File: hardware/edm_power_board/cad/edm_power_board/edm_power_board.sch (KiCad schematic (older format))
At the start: 0 parts

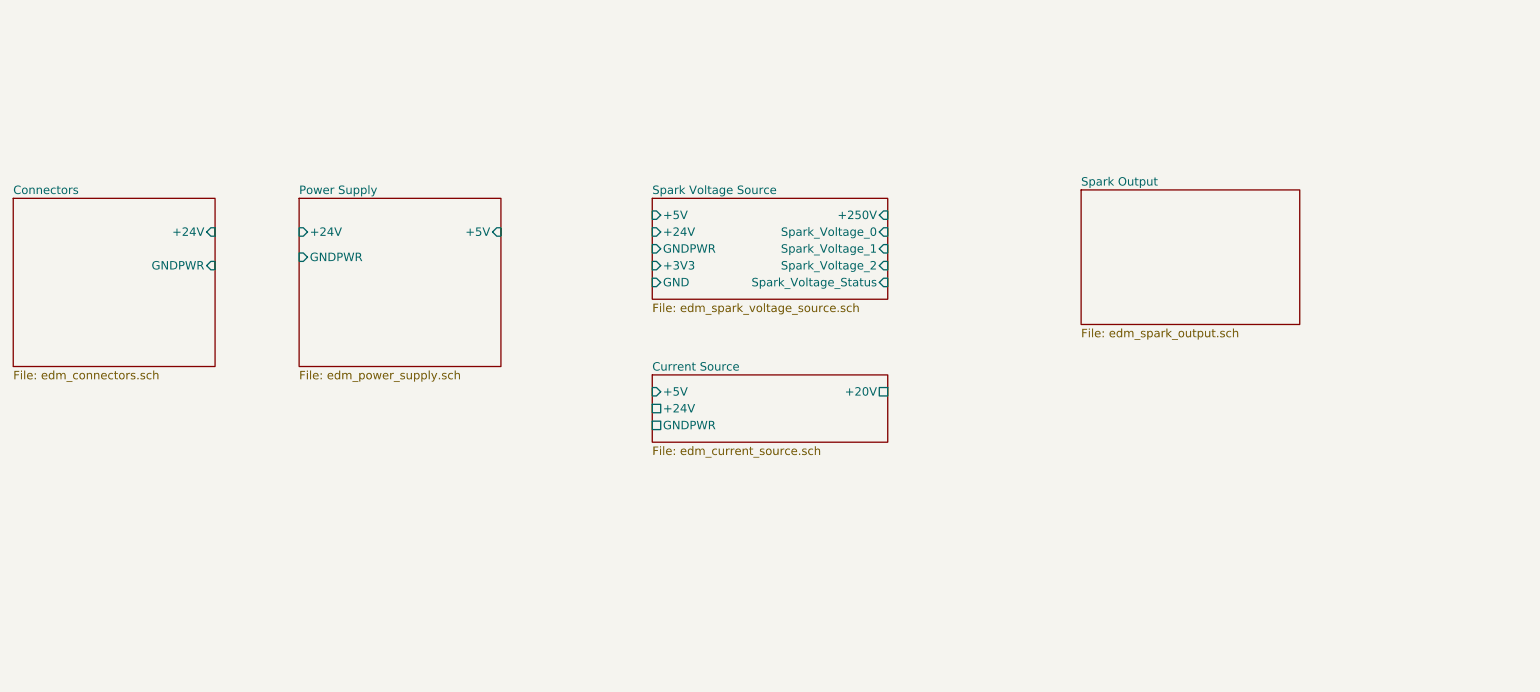
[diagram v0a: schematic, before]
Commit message: Interconnections
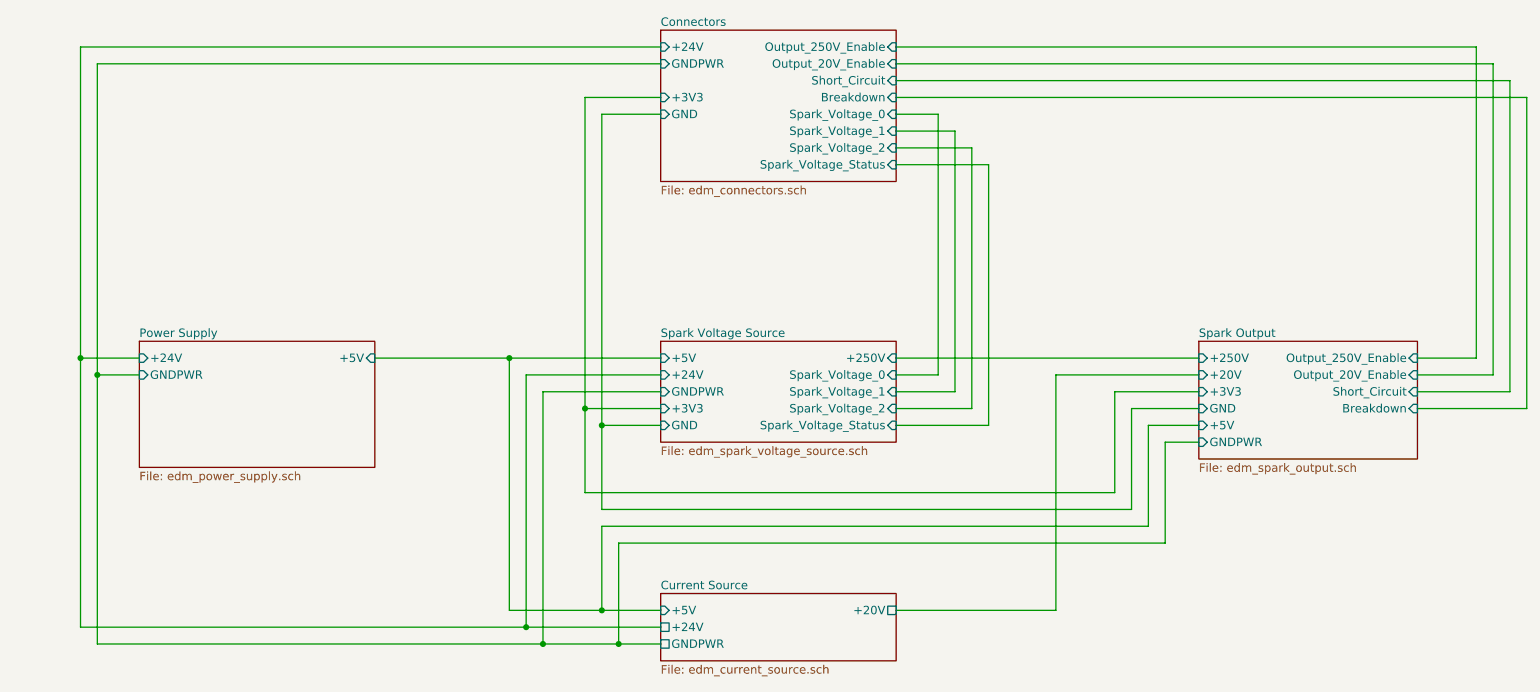
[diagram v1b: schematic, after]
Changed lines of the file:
@@
 $EndDescr
 $Sheet
-S 5000 3750 1400 400
+S 5050 5050 1400 400
 U 5A71F0AB
 F0 "Current Source" 50
 F1 "edm_current_source.sch" 50
-F2 "+24V" U L 5000 3950 50
-F3 "GNDPWR" U L 5000 4050 50
-F4 "+20V" U R 6400 3850 50
-F5 "+5V" I L 5000 3850 50
-$EndSheet
-$Sheet
-S 5000 2700 1400 600
+F2 "+24V" U L 5050 5250 50
+F3 "GNDPWR" U L 5050 5350 50
+F4 "+20V" U R 6450 5150 50
+F5 "+5V" I L 5050 5150 50
+$EndSheet
+$Sheet
+S 5050 3550 1400 600
 U 5A728D61
 F0 "Spark Voltage Source" 50
 F1 "edm_spark_voltage_source.sch" 50
-F2 "+24V" I L 5000 2900 50
-F3 "GNDPWR" I L 5000 3000 50
-F4 "+250V" I R 6400 2800 50
-F5 "+5V" I L 5000 2800 50
-F6 "GND" I L 5000 3200 50
-F7 "+3V3" I L 5000 3100 50
-F8 "Spark_Voltage_0" I R 6400 2900 50
-F9 "Spark_Voltage_1" I R 6400 3000 50
-F10 "Spark_Voltage_2" I R 6400 3100 50
-F11 "Spark_Voltage_Status" I R 6400 3200 50
-$EndSheet
-$Sheet
-S 2900 2700 1200 1000
+F2 "+24V" I L 5050 3750 50
+F3 "GNDPWR" I L 5050 3850 50
+F4 "+250V" I R 6450 3650 50
+F5 "+5V" I L 5050 3650 50
+F6 "GND" I L 5050 4050 50
+F7 "+3V3" I L 5050 3950 50
+F8 "Spark_Voltage_0" I R 6450 3750 50
+F9 "Spark_Voltage_1" I R 6450 3850 50
+F10 "Spark_Voltage_2" I R 6450 3950 50
+F11 "Spark_Voltage_Status" I R 6450 4050 50
+$EndSheet
+$Sheet
+S 1950 3550 1400 750
 U 5A73A880
 F0 "Power Supply" 50
 F1 "edm_power_supply.sch" 50
-F2 "+24V" I L 2900 2900 50
-F3 "GNDPWR" I L 2900 3050 50
-F4 "+5V" I R 4100 2900 50
-$EndSheet
-$Sheet
-S 1200 2700 1200 1000
+F2 "+24V" I L 1950 3650 50
+F3 "GNDPWR" I L 1950 3750 50
+F4 "+5V" I R 3350 3650 50
+$EndSheet
+$Sheet
+S 5050 1700 1400 900
 U 5A73A88E
 F0 "Connectors" 50
 F1 "edm_connectors.sch" 50
-F2 "+24V" I R 2400 2900 50
-F3 "GNDPWR" I R 2400 3100 50
-$EndSheet
-$Sheet
-S 7550 2650 1300 800
+F2 "+24V" I L 5050 1800 50
+F3 "GNDPWR" I L 5050 1900 50
+F4 "Output_250V_Enable" I R 6450 1800 50
+F5 "Output_20V_Enable" I R 6450 1900 50
+F6 "Short_Circuit" I R 6450 2000 50
+F7 "Breakdown" I R 6450 2100 50
+F8 "Spark_Voltage_0" I R 6450 2200 50
+F9 "Spark_Voltage_1" I R 6450 2300 50
+F10 "Spark_Voltage_2" I R 6450 2400 50
+F11 "Spark_Voltage_Status" I R 6450 2500 50
+F12 "+3V3" I L 5050 2100 50
+F13 "GND" I L 5050 2200 50
+$EndSheet
+$Sheet
+S 8250 3550 1300 700
 U 5A9693D9
 F0 "Spark Output" 50
 F1 "edm_spark_output.sch" 50
-$EndSheet
+F2 "+250V" I L 8250 3650 50
+F3 "+20V" I L 8250 3750 50
+F4 "+5V" I L 8250 4050 50
+F5 "+3V3" I L 8250 3850 50
+F6 "GND" I L 8250 3950 50
+F7 "GNDPWR" I L 8250 4150 50
+F8 "Output_250V_Enable" I R 9550 3650 50
+F9 "Output_20V_Enable" I R 9550 3750 50
+F10 "Short_Circuit" I R 9550 3850 50
+F11 "Breakdown" I R 9550 3950 50
+$EndSheet
+Wire Wire Line
+	6450 3650 8250 3650
+Wire Wire Line
+	6450 5150 7400 5150
+Wire Wire Line
+	7400 5150 7400 3750
+Wire Wire Line
+	7400 3750 8250 3750
+Wire Wire Line
+	6450 3750 6700 3750
+Wire Wire Line
+	6700 3750 6700 2200
+Wire Wire Line
+	6700 2200 6450 2200
+Wire Wire Line
+	6450 2300 6800 2300
+Wire Wire Line
+	6800 2300 6800 3850
+Wire Wire Line
+	6800 3850 6450 3850
+Wire Wire Line
+	6450 3950 6900 3950
+Wire Wire Line
+	6900 3950 6900 2400
+Wire Wire Line
+	6900 2400 6450 2400
+Wire Wire Line
+	6450 2500 7000 2500
+Wire Wire Line
+	7000 2500 7000 4050
+Wire Wire Line
+	7000 4050 6450 4050
+Wire Wire Line
+	6450 2100 10200 2100
+Wire Wire Line
+	10200 2100 10200 3950
+Wire Wire Line
+	10200 3950 9550 3950
+Wire Wire Line
+	6450 2000 10100 2000
+Wire Wire Line
+	10100 2000 10100 3850
+Wire Wire Line
+	10100 3850 9550 3850
+Wire Wire Line
+	9550 3750 10000 3750
+Wire Wire Line
+	10000 3750 10000 1900
+Wire Wire Line
+	10000 1900 6450 1900
+Wire Wire Line
+	6450 1800 9900 1800
+Wire Wire Line
+	9900 1800 9900 3650
+Wire Wire Line
+	9900 3650 9550 3650
+Wire Wire Line
+	3350 3650 4150 3650
+Wire Wire Line
+	5050 5150 4700 5150
+Wire Wire Line
+	4150 5150 4150 3650
+Connection ~ 4150 3650
+Wire Wire Line
+	4150 3650 5050 3650
+Wire Wire Line
+	5050 5250 4250 5250
+Wire Wire Line
+	4250 5250 4250 3750
+Wire Wire Line
+	4250 3750 5050 3750
+Wire Wire Line
+	5050 3850 4350 3850
+Wire Wire Line
+	4350 3850 4350 5350
+Wire Wire Line
+	4350 5350 4800 5350
+Wire Wire Line
+	5050 3950 4600 3950
+Wire Wire Line
+	4600 3950 4600 2100
+Wire Wire Line
+	4600 2100 5050 2100
+Wire Wire Line
+	5050 4050 4700 4050
+Wire Wire Line
+	4700 4050 4700 2200
+Wire Wire Line
+	4700 2200 5050 2200
+Wire Wire Line
+	7750 4450 4600 4450
+Wire Wire Line
+	4600 4450 4600 3950
+Connection ~ 4600 3950
+Wire Wire Line
+	7850 4550 4700 4550
+Wire Wire Line
+	4700 4550 4700 4050
+Connection ~ 4700 4050
+Wire Wire Line
+	4350 5350 1700 5350
+Wire Wire Line
+	1700 5350 1700 3750
+Wire Wire Line
+	1700 3750 1950 3750
+Connection ~ 4350 5350
+Wire Wire Line
+	1950 3650 1600 3650
+Wire Wire Line
+	1600 3650 1600 5250
+Wire Wire Line
+	1600 5250 4250 5250
+Connection ~ 4250 5250
+Wire Wire Line
+	4800 5350 4800 4750
+Connection ~ 4800 5350
+Wire Wire Line
+	4800 5350 5050 5350
+Wire Wire Line
+	4700 4650 4700 5150
+Connection ~ 4700 5150
+Wire Wire Line
+	4700 5150 4150 5150
+Wire Wire Line
+	7750 4450 7750 3850
+Wire Wire Line
+	7750 3850 8250 3850
+Wire Wire Line
+	8250 3950 7850 3950
+Wire Wire Line
+	7850 3950 7850 4550
+Wire Wire Line
+	8250 4050 7950 4050
+Wire Wire Line
+	7950 4050 7950 4650
+Wire Wire Line
+	4700 4650 7950 4650
+Wire Wire Line
+	8050 4750 8050 4150
+Wire Wire Line
+	8050 4150 8250 4150
+Wire Wire Line
+	4800 4750 8050 4750
+Wire Wire Line
+	1700 3750 1700 1900
+Wire Wire Line
+	1700 1900 5050 1900
+Connection ~ 1700 3750
+Wire Wire Line
+	5050 1800 1600 1800
+Wire Wire Line
+	1600 1800 1600 3650
+Connection ~ 1600 3650
 $EndSCHEMATC
